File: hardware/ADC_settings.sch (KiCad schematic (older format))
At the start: 10 parts

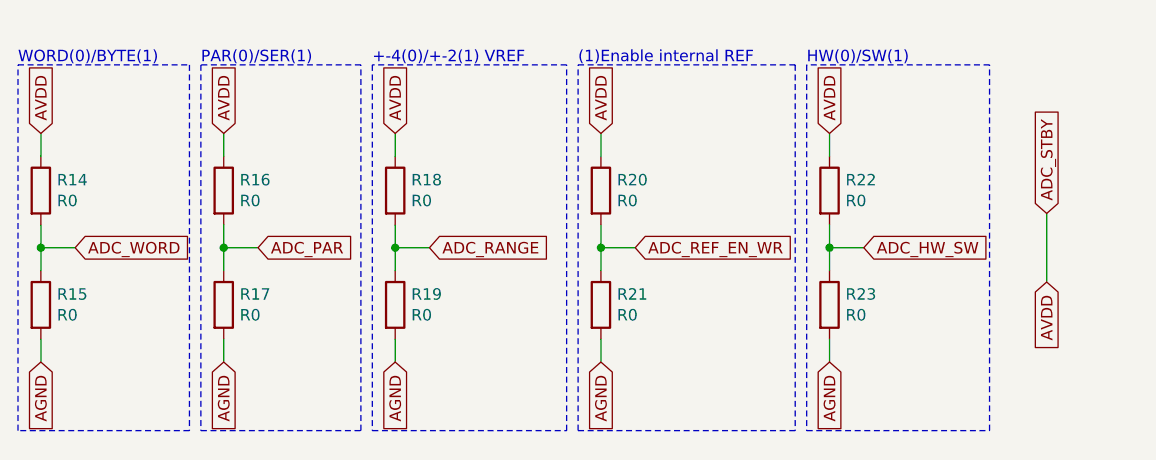
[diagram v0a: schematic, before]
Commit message: Adding last known changes to shematics
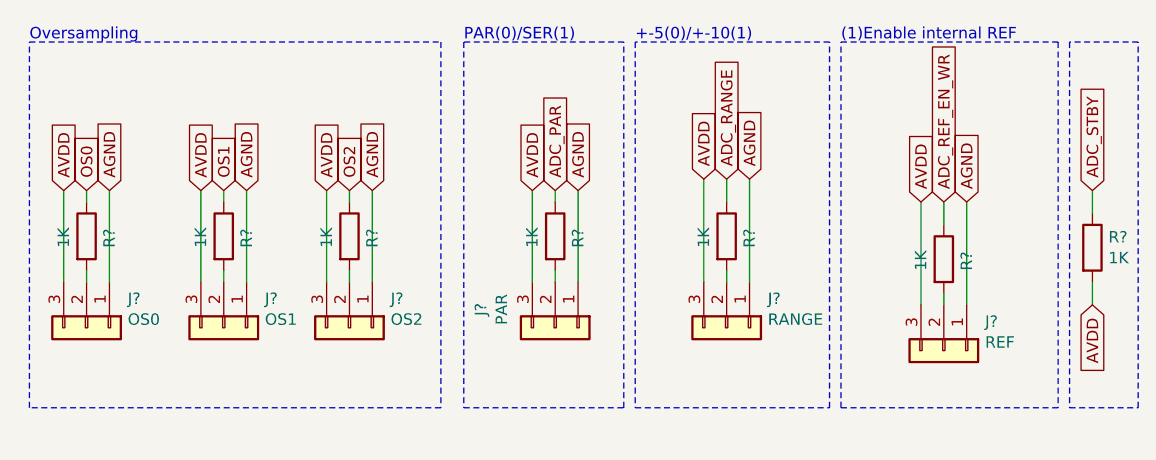
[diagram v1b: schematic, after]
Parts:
- removed R14, R15, R16, R17, R18, R19, R20, R21, R22, R23: R0, Resistor_SMD:R_0805_2012Metric, symbol antena:R
- added J?: PAR, symbol Connector_Generic:Conn_01x03
- added J?: RANGE, symbol Connector_Generic:Conn_01x03
- added J?: REF, symbol Connector_Generic:Conn_01x03
- added J?: OS0, symbol Connector_Generic:Conn_01x03
- added J?: OS1, symbol Connector_Generic:Conn_01x03
- added J?: OS2, symbol Connector_Generic:Conn_01x03
- added R? (x7): 1K, Resistor_SMD:R_0805_2012Metric, symbol antena:R
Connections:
- net ADC_PAR: now also R?.1
- net ADC_RANGE: now also R?.1
- net ADC_REF_EN_WR: now also R?.1
- net ADC_STBY: now also R?.1
- net AGND: now also J?.1 (Pin_1), J?.1 (Pin_1), J?.1 (Pin_1), J?.1 (Pin_1), J?.1 (Pin_1), J?.1 (Pin_1)
- new net: J?.2 (Pin_2), R?.2 (x6)
- new net AVDD: J?.3 (Pin_3), J?.3 (Pin_3), J?.3 (Pin_3), J?.3 (Pin_3), J?.3 (Pin_3), J?.3 (Pin_3), R?.2
- new net OS0: R?.1
- new net OS1: R?.1
- new net OS2: R?.1
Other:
- note added: "+-5(0)/+-10(1)"
- note added: "Oversampling"
- note removed: "+-4(0)/+-2(1) VREF"
- note removed: "HW(0)/SW(1)"
- note removed: "WORD(0)/BYTE(1)"
